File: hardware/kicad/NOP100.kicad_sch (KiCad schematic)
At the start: 45 parts, among them CON1 CLICK MODULE 0, CON2 CLICK MODULE 1, J1 CAN, Q1 BSS138, Q2 BSS138, SW1 BUS, SW2 SW_Push, U1 MURATA_MEJ2*, U2 MCP2551-I-P, U3 Teensy_4.0, U4 74HC165, U6 NCS1S1203SC

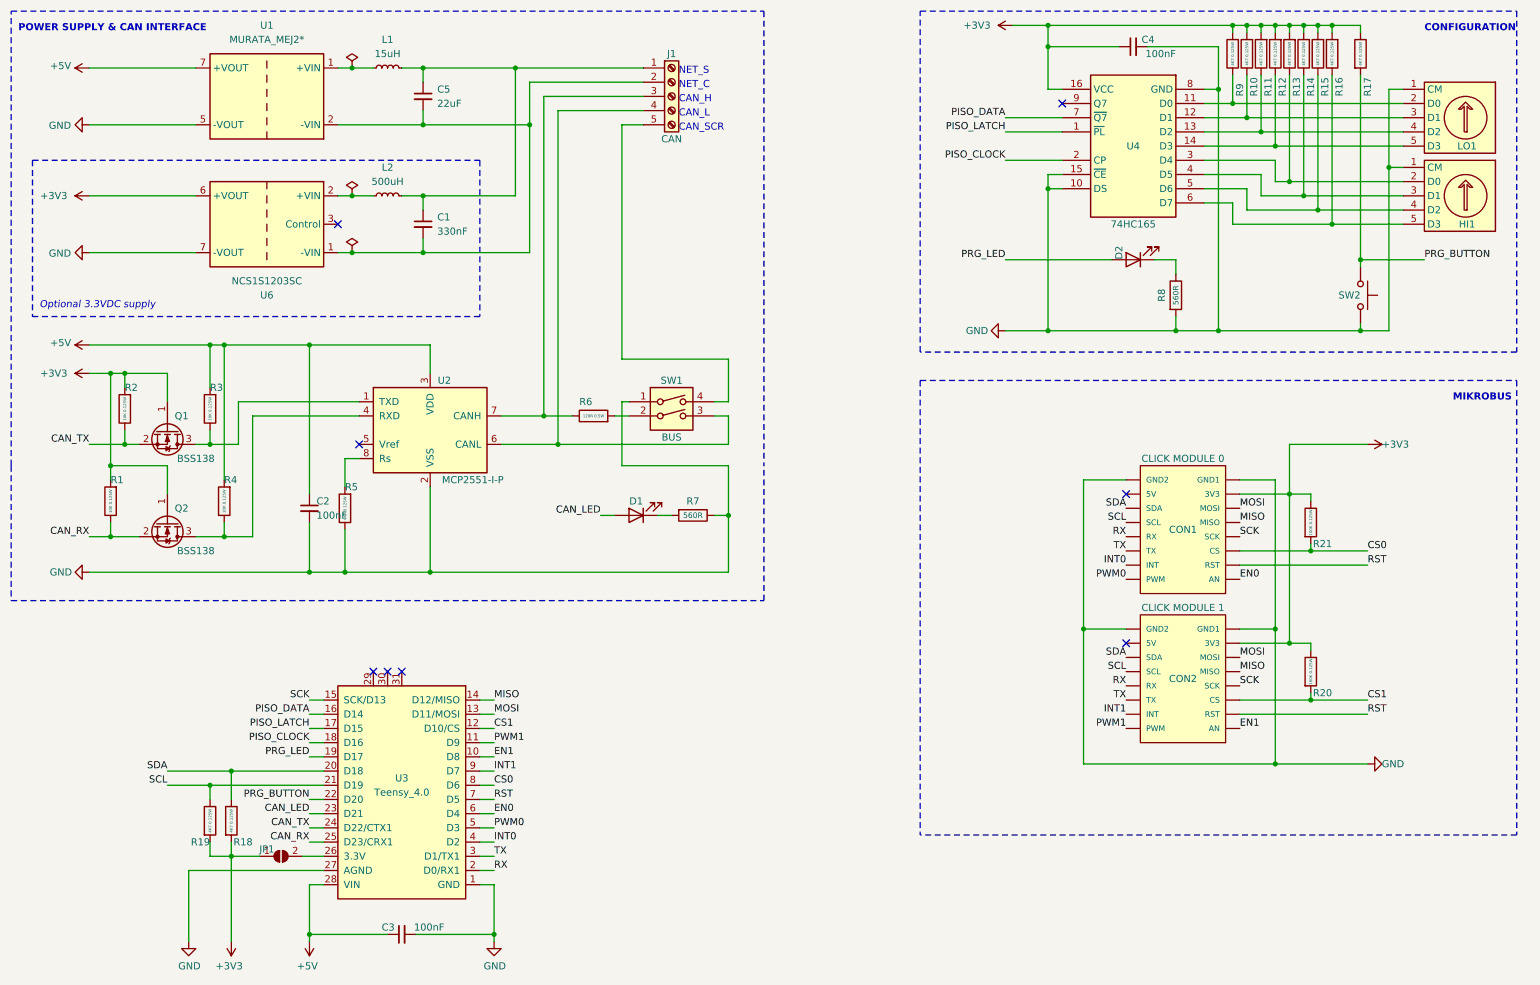
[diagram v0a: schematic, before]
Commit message: Tweaks
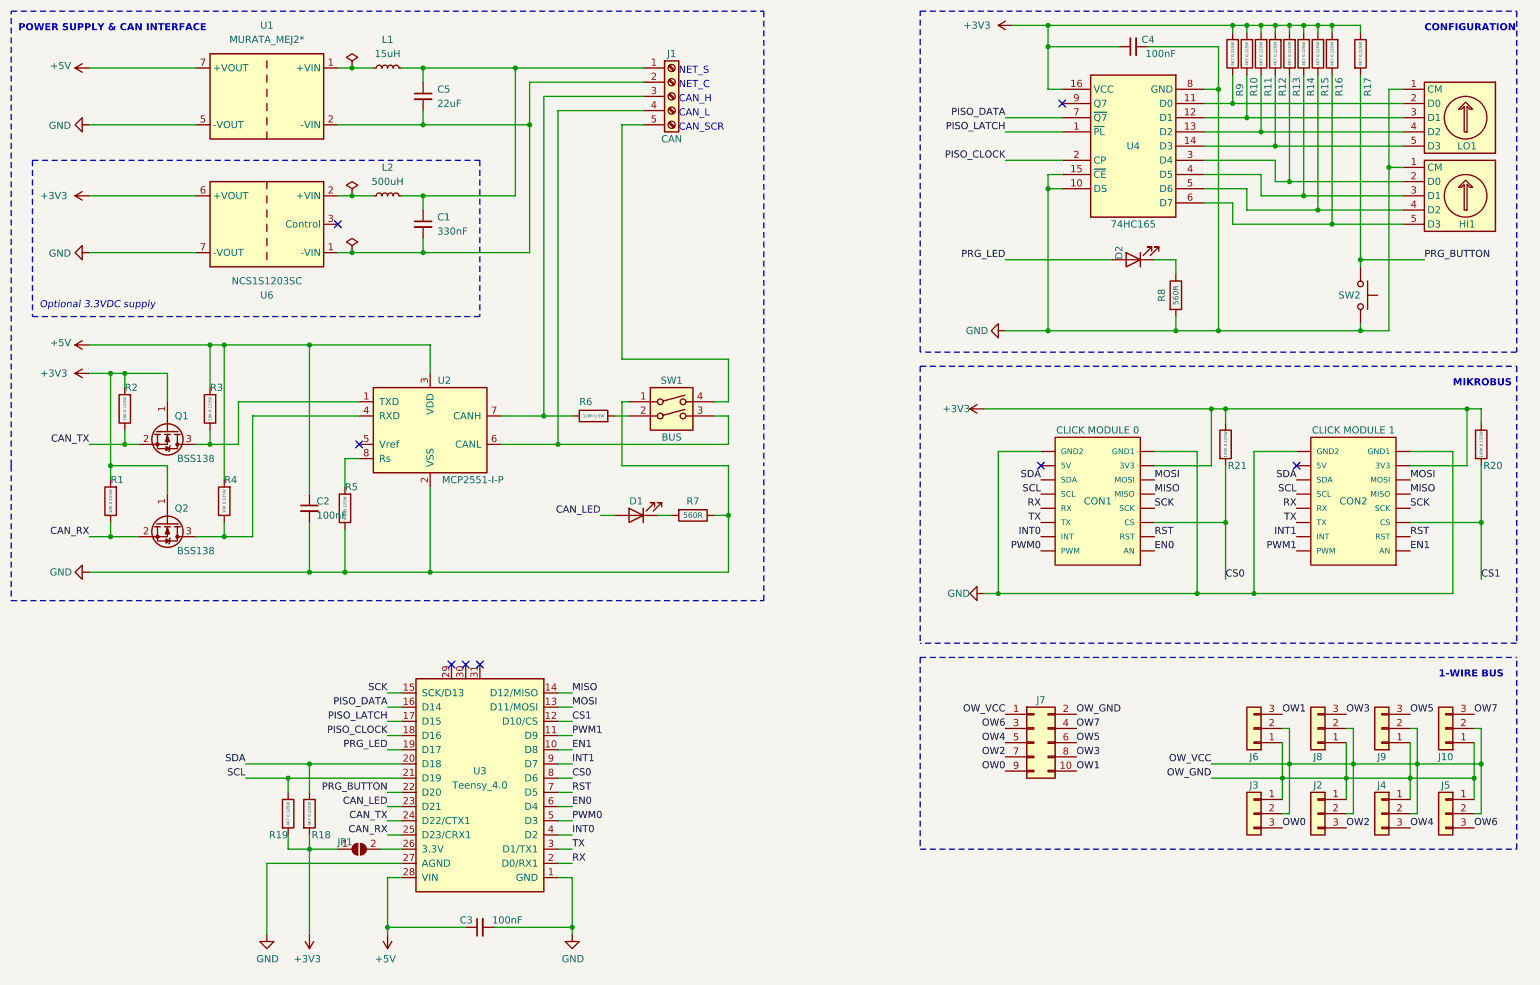
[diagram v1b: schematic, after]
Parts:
- added J10, J2, J3, J4, J5, J6, J8, J9: Conn_01x03, pdjr:RS_8971054, symbol Connector_Generic:Conn_01x03
- added J7: Conn_02x05_Odd_Even, Connector_PinSocket_2.54mm:PinSocket_2x05_P2.54mm_Vertical, symbol Connector_Generic:Conn_02x05_Odd_Even
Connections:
- new net OW0: J3.3 (Pin_3), J7.9 (Pin_9)
- new net OW1: J6.3 (Pin_3), J7.10 (Pin_10)
- new net OW2: J2.3 (Pin_3), J7.7 (Pin_7)
- new net OW3: J7.8 (Pin_8), J8.3 (Pin_3)
- new net OW4: J4.3 (Pin_3), J7.5 (Pin_5)
- new net OW5: J7.6 (Pin_6), J9.3 (Pin_3)
- new net OW6: J5.3 (Pin_3), J7.3 (Pin_3)
- new net OW7: J10.3 (Pin_3), J7.4 (Pin_4)
- new net OW_GND: J10.1 (Pin_1), J2.1 (Pin_1), J3.1 (Pin_1), J4.1 (Pin_1), J5.1 (Pin_1), J6.1 (Pin_1), J7.2 (Pin_2), J8.1 (Pin_1), J9.1 (Pin_1)
- new net OW_VCC: J10.2 (Pin_2), J2.2 (Pin_2), J3.2 (Pin_2), J4.2 (Pin_2), J5.2 (Pin_2), J6.2 (Pin_2), J7.1 (Pin_1), J8.2 (Pin_2), J9.2 (Pin_2)
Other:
- note added: "1-WIRE BUS"
- moved on the sheet: C3, CON1, CON2, JP1, R18, R19, R20, R21, U3
